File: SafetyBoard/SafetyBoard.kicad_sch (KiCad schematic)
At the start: 18 parts, among them J1 Estop, J2 TS ON SW, J3 SDC OUT, J4 ACCU, J5 12v EXP, J6 PWR IN, J7 24v EXP, J8 5v EXP

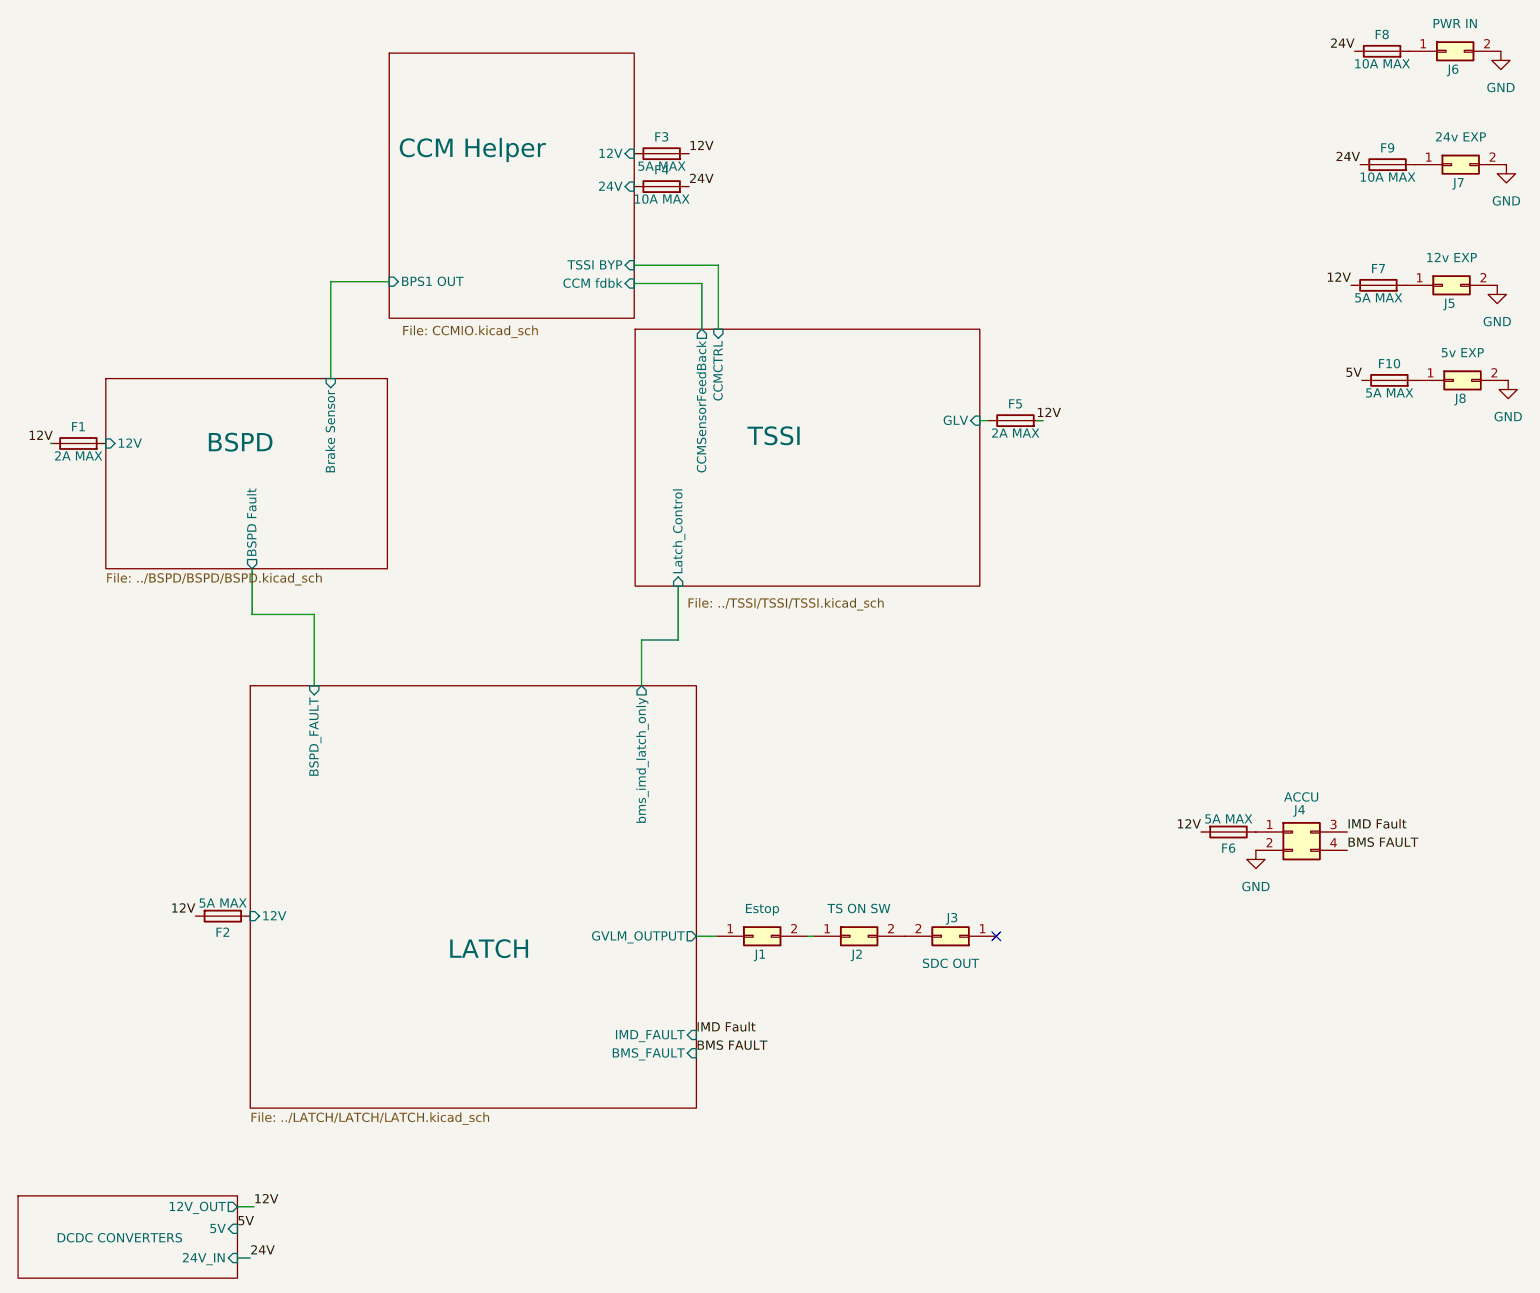
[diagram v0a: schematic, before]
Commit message: updates I think
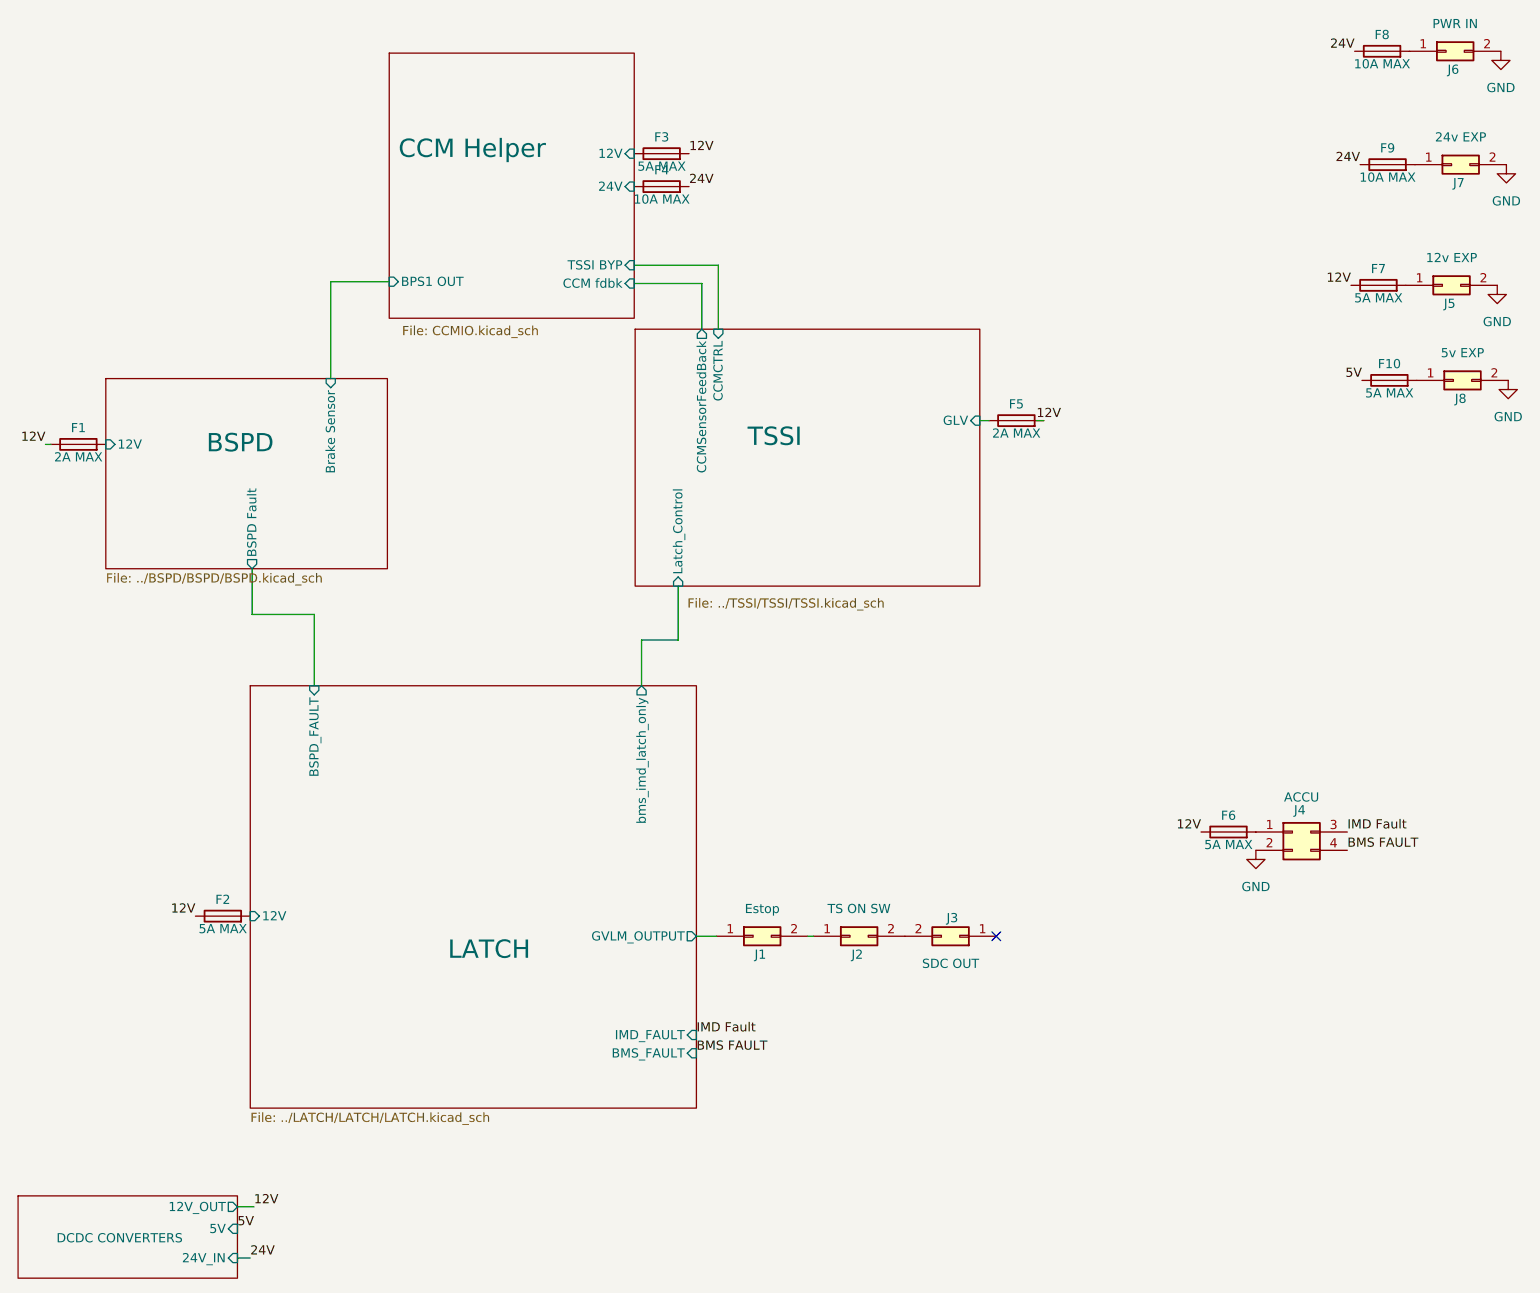
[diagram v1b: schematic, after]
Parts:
- F1, F10, F2, F5, F6, F7, F8, F9: MFG Littelfuse -> Keystone Electronics; MPN 01530007Z -> 3522-2
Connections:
- net 12V: now also F2.1, F6.1; no longer F2.2, F6.2
- net LATCH/12V: now also F2.2; no longer F2.1
- net at J4.1 (Pin_1): now also F6.2; no longer F6.1
